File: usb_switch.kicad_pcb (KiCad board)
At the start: 2 copper layers, 67 parts, among them CON1 2_Post_Terminal, CON2 2_Post_Terminal, CON3 2_Post_Terminal, CON4 2_Post_Terminal, CON5 2_Post_Terminal, CON6 2_Post_Terminal, U1 AP2120N, U2 STM32F042K6T6, U3 Si1869DH, U4 Si1869DH, U5 Si1869DH, U6 Si1869DH, U7 Si1869DH, U8 Si1869DH

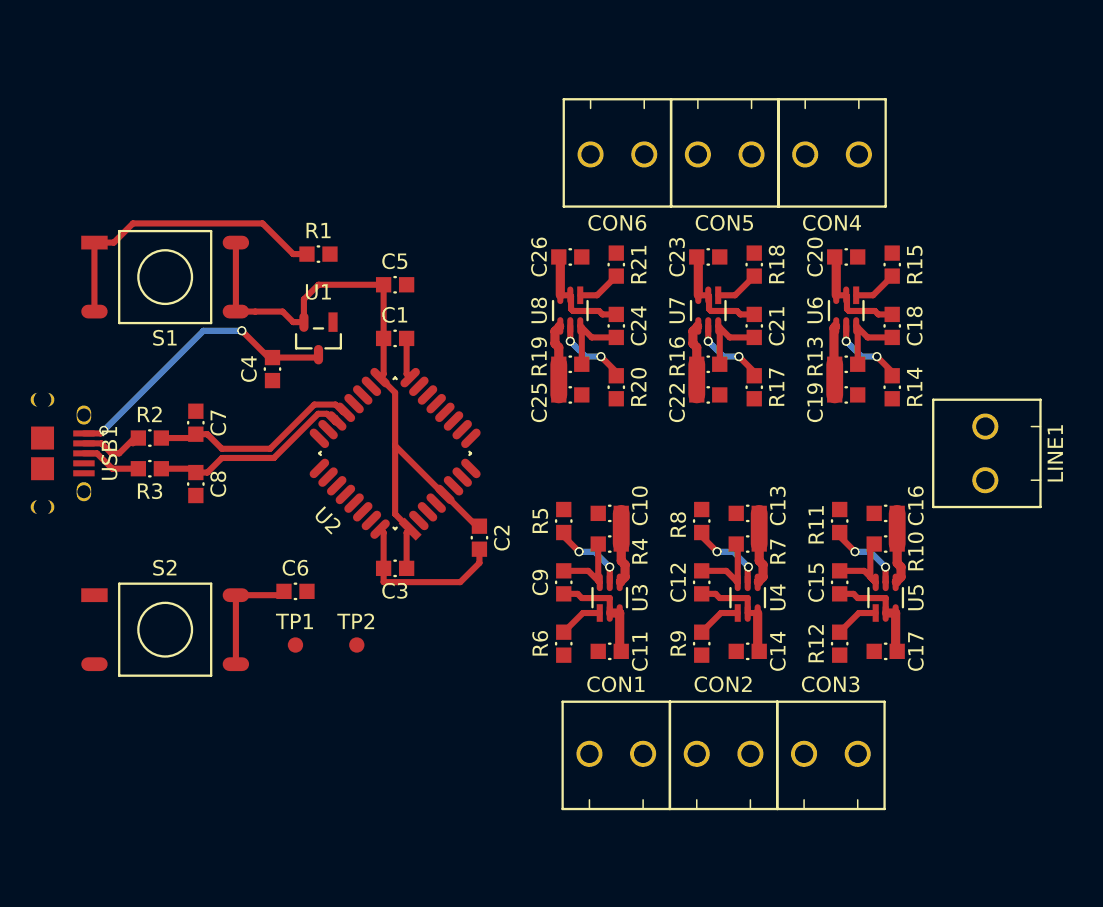
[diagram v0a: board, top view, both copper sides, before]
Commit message: Finish routing the PCB.
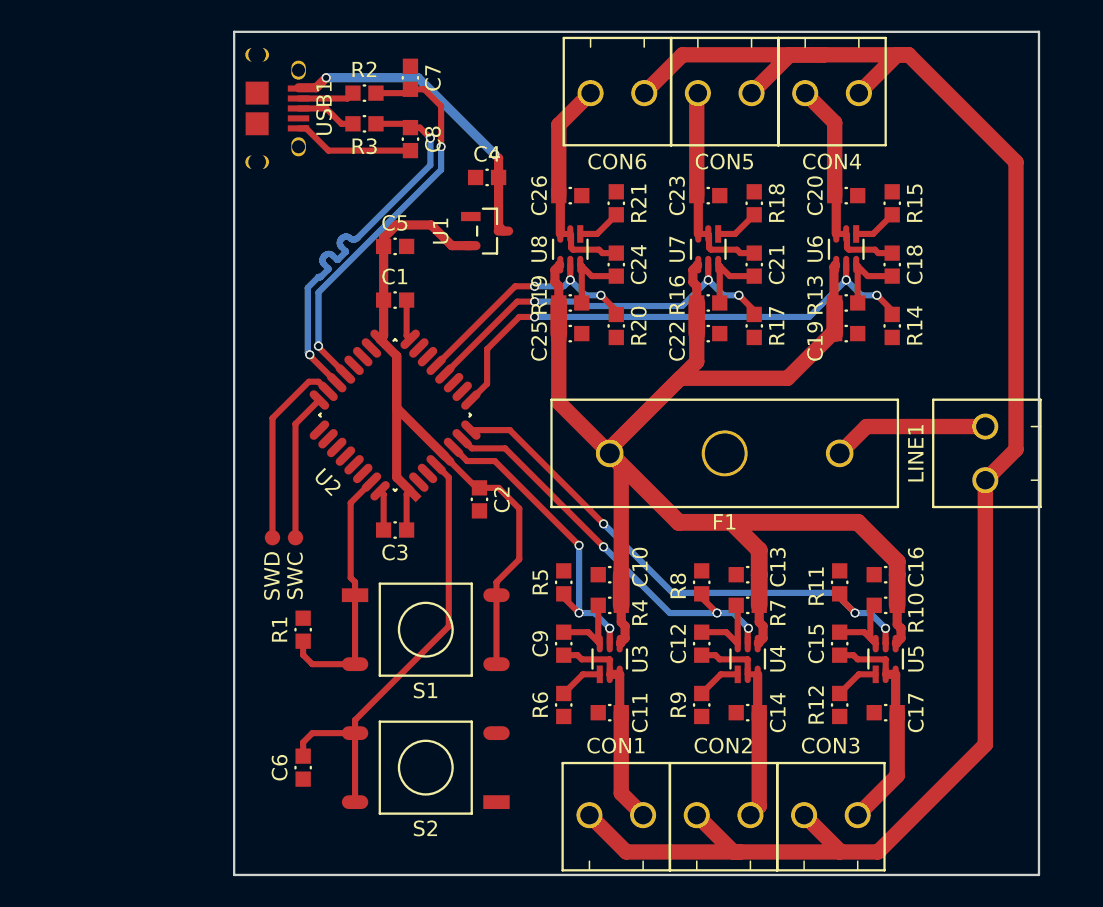
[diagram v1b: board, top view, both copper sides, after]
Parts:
- added F1: 2A, parts:Fuse_Block, F.Cu at (145.9, 89.4)
- moved S1 28.6 mm to (126.4, 100.9)
- moved C7 26.5 mm to (125.4, 64.9)
- moved C8 26.5 mm to (125.4, 68.9)
- moved R2 26.5 mm to (122.4, 65.9)
- moved R3 26.5 mm to (122.4, 67.9)
- moved USB1 26.5 mm to (115.4, 66.9)
- moved R1 24.5 mm to (118.4, 100.9), turned to 270 degrees
- moved S2 19.2 mm to (126.4, 109.9), turned to 180 degrees
- moved C4 18.8 mm to (130.4, 71.4), turned to 0 degrees
- moved U1 13.0 mm to (130.4, 74.9), turned to 0 degrees
- moved C6 11.5 mm to (118.4, 109.9), turned to 270 degrees
- moved TP2 8.06 mm to (117.9, 94.9)
- moved TP1 7.16 mm to (116.4, 94.9)
- moved C10 4.00 mm to (138.4, 97.3)
- moved C11 4.00 mm to (138.4, 106.3)
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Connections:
- LINE1 pad 1: Line -> Net-(F1-Pad1)
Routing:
- net GND: track 13.9 -> 127.2 mm
- net Line: track 28.2 -> 100.8 mm
- net /Switch 3/SW: track 5.07 -> 35.1 mm, vias 2 -> 3
- net /Switch 4/SW: track 5.08 -> 34.1 mm, vias 2 -> 3
- net Net-(C6-Pad1): track 7.74 -> 29.4 mm
- net /Switch 2/SW: track 5.15 -> 26.5 mm, vias 2 -> 3
- net /Switch 5/SW: track 5.08 -> 25.0 mm, vias 2 -> 3
- net /Switch 1/SW: track 5.08 -> 20.3 mm, vias 2 -> 3
- net /USB_D-: track 13.7 -> 26.6 mm, vias 0 -> 2
- net Net-(TP1-Pad1): track 0.00 -> 12.7 mm
- net /USB_D+: track 14.2 -> 26.6 mm, vias 0 -> 2
- net /Switch 6/SW: track 5.08 -> 16.1 mm, vias 2 -> 3
- net Net-(F1-Pad1): track 0.00 -> 10.2 mm
- net Net-(TP2-Pad1): track 0.00 -> 9.63 mm
- net +3.3V: track 43.5 -> 51.6 mm
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- added copper zone on B.Cu, net GND
- added copper zone on F.Cu, net GND
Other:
- board outline added: 52.5 x 55 mm
